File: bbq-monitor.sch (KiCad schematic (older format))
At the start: 51 parts, among them J1 Power, J2 USB_B_Mini, J3 Thermocouple, Q1 AO3401A, Q2 BC847, Q3 BC847, SW1 SW_Push, U1 ESP32-WROOM-32D, U2 TPS62132, U3 CP2104, U4 USBLC6-2SC6, U5 AD8495, U6 DHT11

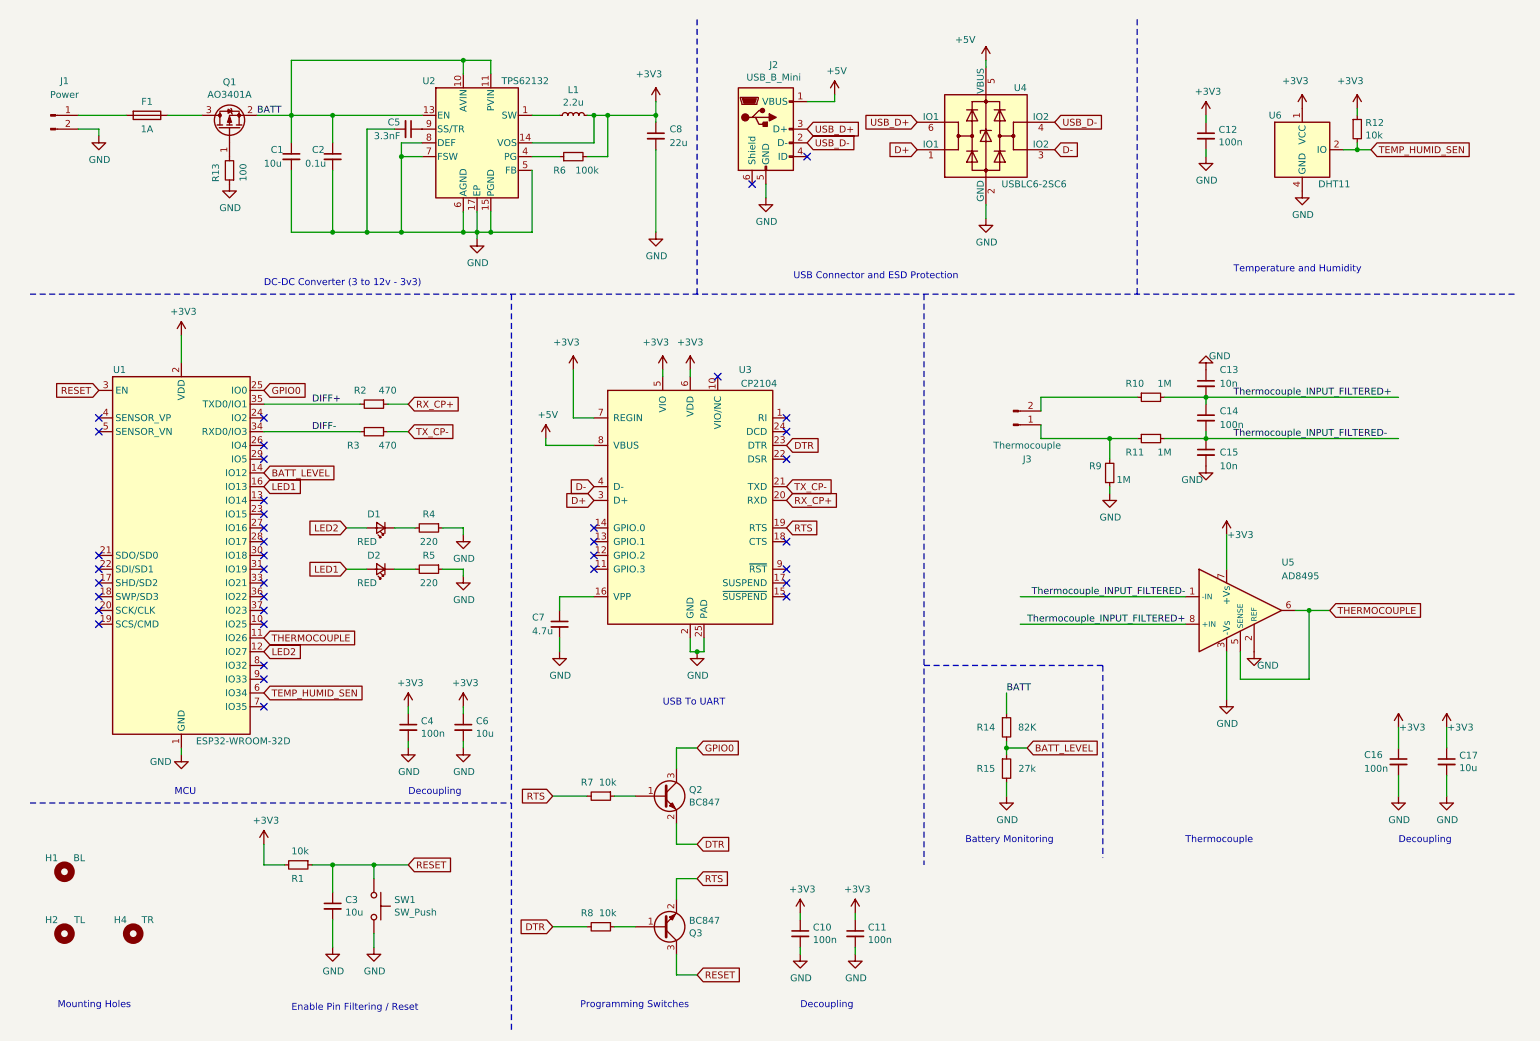
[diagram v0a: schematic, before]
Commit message: up
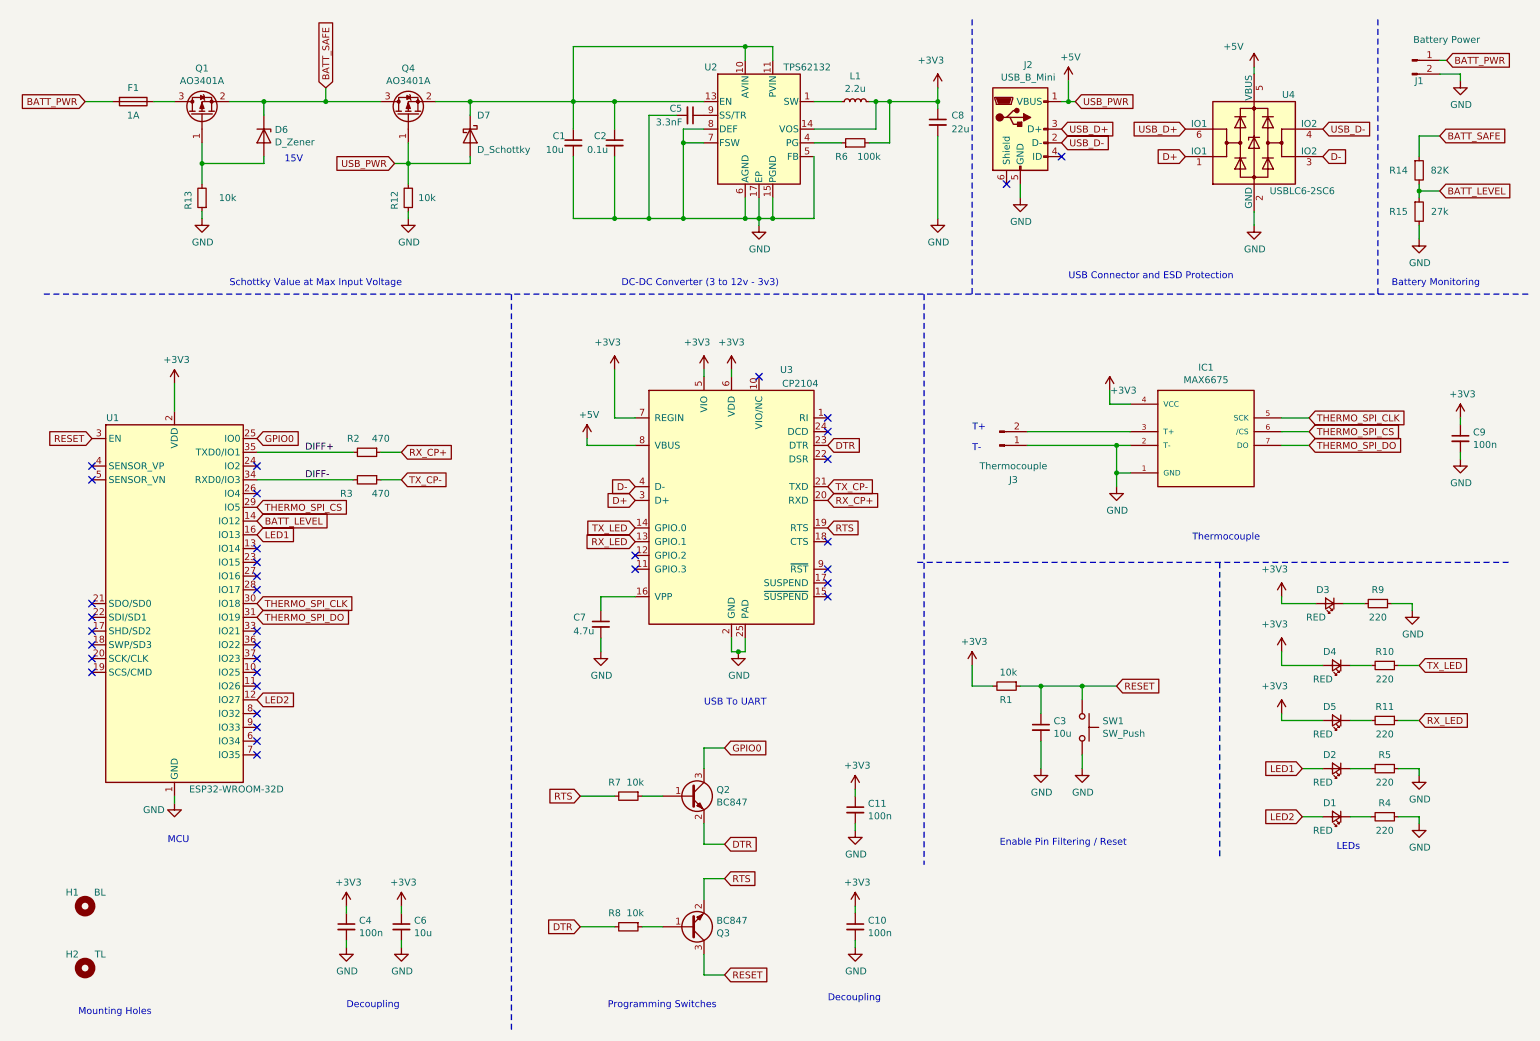
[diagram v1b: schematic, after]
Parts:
- removed C12, C14: 100n, Capacitor_SMD:C_0603_1608Metric, symbol Device:C_Small
- removed C13, C15: 10n, Capacitor_SMD:C_0603_1608Metric, symbol Device:C_Small
- removed C16: 100n, Capacitor_SMD:C_0402_1005Metric, symbol Device:C_Small
- removed C17: 10u, Capacitor_SMD:C_0402_1005Metric, symbol Device:C_Small
- removed H4: TR, MountingHole:MountingHole_3.2mm_M3_Pad_Via, symbol Mechanical:MountingHole
- removed U5: AD8495, Package_SO:MSOP-8_3x3mm_P0.65mm, symbol Sensor_Temperature:AD8495
- removed U6: DHT11, Sensor:Aosong_DHT11_5.5x12.0_P2.54mm, symbol Sensor:DHT11
- added C9: 100n, Capacitor_SMD:C_0603_1608Metric, symbol Device:C_Small
- added D3, D4, D5: RED, LED_SMD:LED_0603_1608Metric, symbol Device:LED_Small
- added D6: D_Zener, Diode_SMD:D_1206_3216Metric, symbol Device:D_Zener
- added D7: D_Schottky, Diode_SMD:D_1206_3216Metric, symbol Device:D_Schottky
- added IC1: MAX6675, hardware libraries:SO08, symbol MAX6675:MAX6675
- added Q4: AO3401A, Package_TO_SOT_SMD:SOT-23, symbol Transistor_FET:AO3401A
- J1: value Power -> Battery Power
- R10, R11, R9: value 1M -> 220; LCSC Part # C4190 -> (none)
- R13: value 100 -> 10k
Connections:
- net +3V3: now also C9.1, D3.2 (A), D4.2 (A), D5.2 (A), IC1.4 (VCC); no longer R12.1
- net +5V: now also R12.2, D7.2 (A), Q4.1 (G)
- net GND: now also J3.1 (Pin_1), R12.1, C9.2, IC1.1 (GND), IC1.2 (T-)
- net THERMO_SPI_CS: now reaches U1.29 (IO5)
- net THERMO_SPI_CS: now also IC1.6 (/CS)
- net THERMO_SPI_CLK: now reaches U1.30 (IO18)
- net THERMO_SPI_CLK: now also IC1.5 (SCK)
- net THERMO_SPI_DO: now reaches U1.31 (IO19)
- net THERMO_SPI_DO: now also IC1.7 (DO)
- net RX_LED: now reaches U3.13 (GPIO.1)
- net RX_LED: now also R11.1
- net TX_LED: now reaches U3.14 (GPIO.0)
- net TX_LED: now also R10.1
- net BATT_PWR: now reaches F1.2, J1.1 (Pin_1)
- net at Q1.1 (G), R13.2: now also D6.2 (A)
- net at J3.2 (Pin_2): now also IC1.3 (T+); no longer R10.1
- net BATT: no longer names the net of C1.1, C2.1, U2.10 (AVIN), U2.11 (PVIN), U2.12 (PVIN), U2.13 (EN)
- net BATT: now also D7.1 (K), Q4.2 (S); no longer Q1.2 (S), R14.1
- net TEMP_HUMID_SEN: no longer names the net of U1.6 (IO34)
- net TEMP_HUMID_SEN: no longer R12.2
- net THERMOCOUPLE: no longer names the net of U1.11 (IO26)
- net Thermocouple_INPUT_FILTERED+: no longer names the net of R10.2
- net Thermocouple_INPUT_FILTERED+: now also D4.1 (K)
- net Thermocouple_INPUT_FILTERED-: no longer names the net of R11.2
- net Thermocouple_INPUT_FILTERED-: now also D5.1 (K)
- new net: D3.1 (K), R9.2
- new net BATT_SAFE: D6.1 (K), Q1.2 (S), Q4.3 (D), R14.1
- no-connect marks 38 -> 35
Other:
- note added: "15V"
- note added: "LEDs\n"
- note added: "Schottky Value at Max Input Voltage"
- note added: "T+\n"
- note added: "T-\n"
- note removed: "Temperature and Humidity\n"
- moved on the sheet: C1, C10, C11, C2, C3, C4, C5, C6, C7, C8, D1, D2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
